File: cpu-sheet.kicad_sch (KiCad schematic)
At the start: 52 parts, among them J3 GPIO_HEADER, J4 GPIOR_HEADER, J5 USB_B_Micro, J6 PROG_CONN, U11 CH340G, U6 SRV05-4, U7 23LC1024, U8 STM32L432KC, U9 SRV05-4, Y2 32.768K, Y3 12M

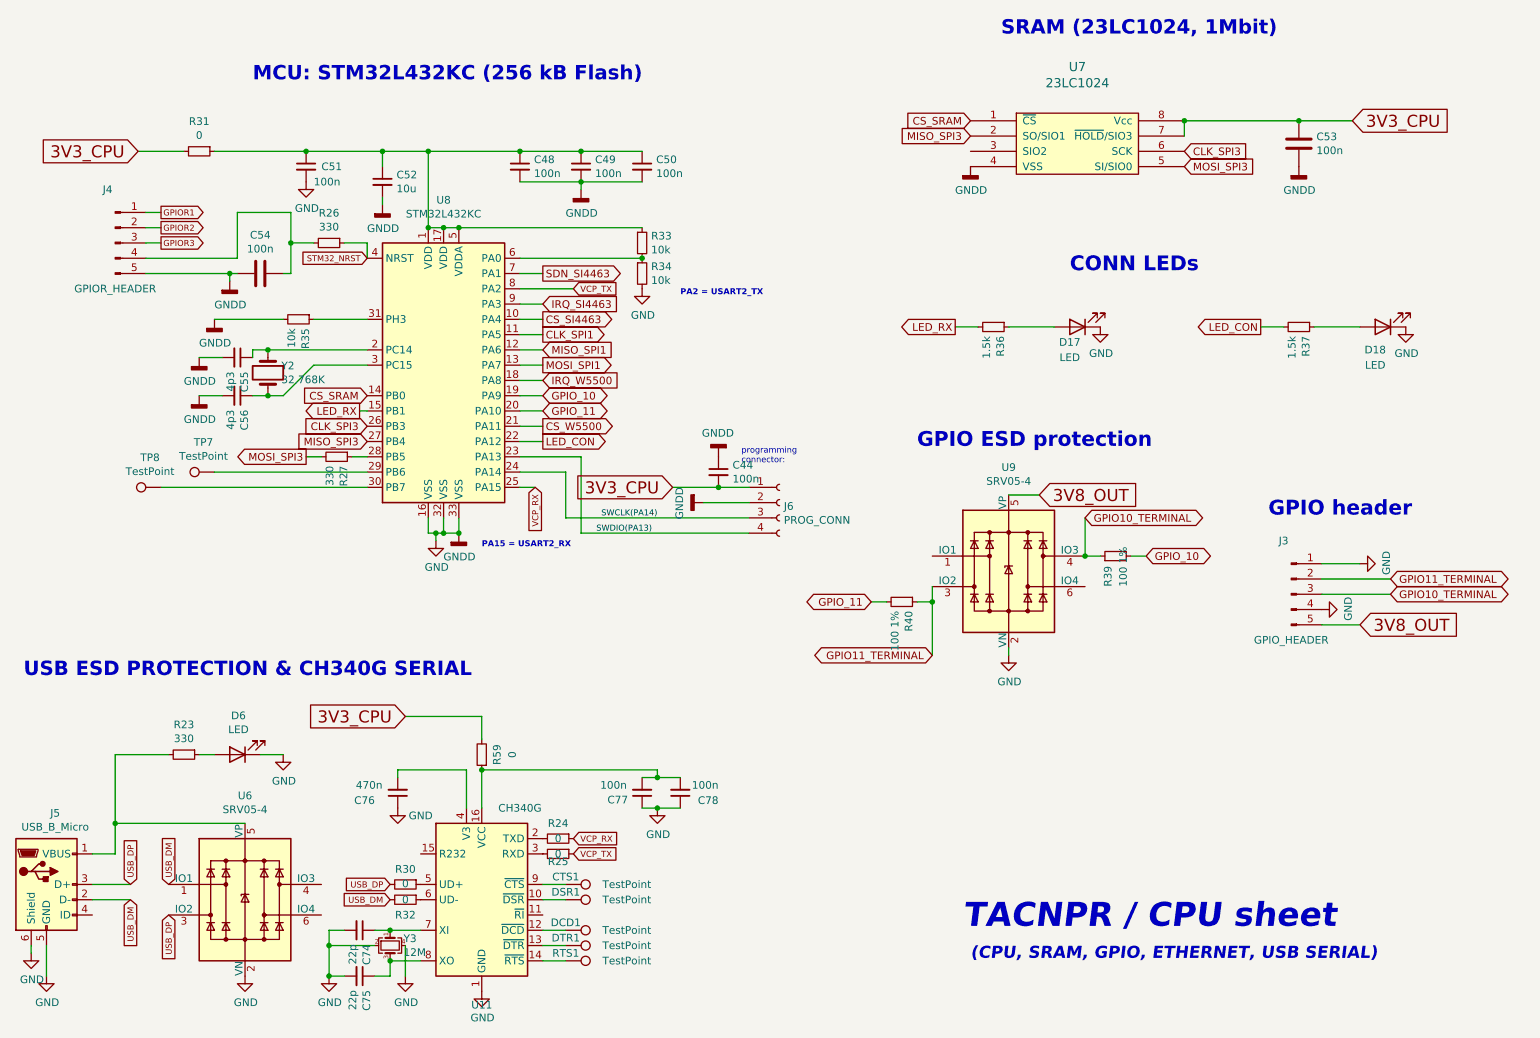
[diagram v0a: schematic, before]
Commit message: misc
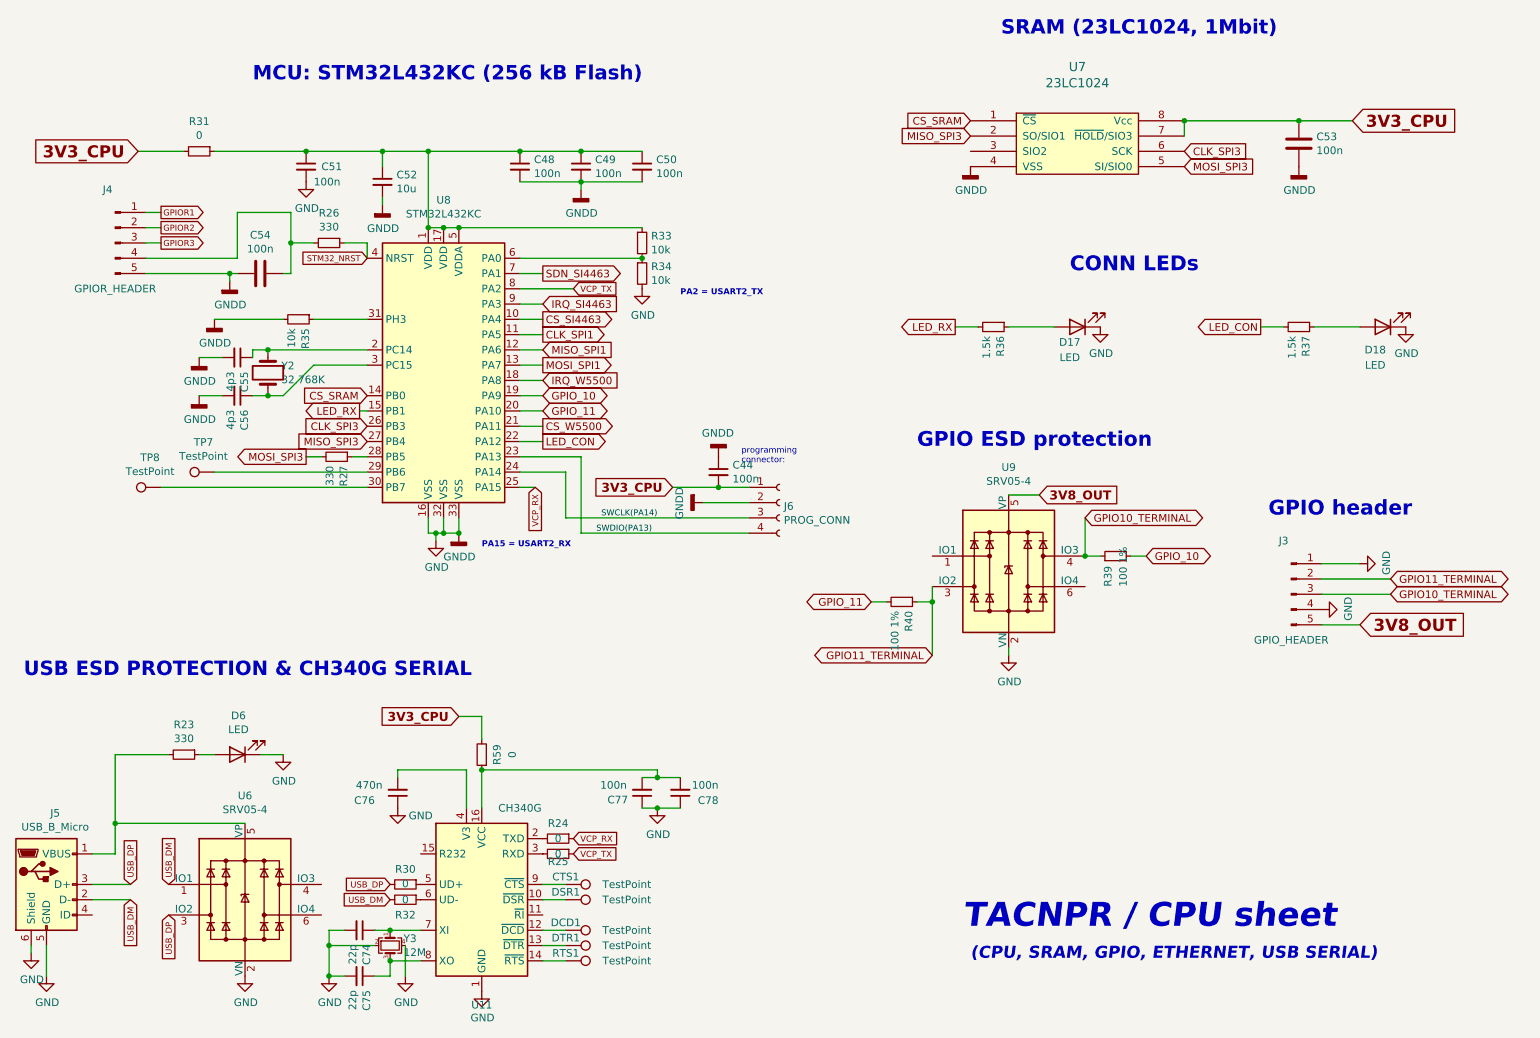
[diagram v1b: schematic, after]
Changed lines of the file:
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@@
     (stroke (width 0) (type default) (color 0 0 0 0))
   )
-  (wire (pts (xy 91.44 138.43) (xy 104.14 138.43))
+  (wire (pts (xy 100.33 138.43) (xy 104.14 138.43))
     (stroke (width 0) (type default) (color 0 0 0 0))
   )
@@
   )
   (global_label "3V3_CPU" (shape input) (at 248.92 39.37 0) (fields_autoplaced)
-    (effects (font (size 2.0066 2.0066)) (justify left))
-    (property "Intersheet References" "${INTERSHEET_REFS}" (id 0) (at 0 0 0)
-      (effects (font (size 1.27 1.27)) hide)
+    (effects (font (size 2.0066 2.0066) (thickness 0.4013) bold) (justify left))
+    (property "Intersheet References" "${INTERSHEET_REFS}" (id 0) (at 266.0792 39.1694 0)
+      (effects (font (size 2.0066 2.0066) (thickness 0.4013) bold) (justify left) hide)
     )
   )
@@
   )
   (global_label "3V8_OUT" (shape input) (at 250.19 123.19 0) (fields_autoplaced)
-    (effects (font (size 2.0066 2.0066)) (justify left))
-    (property "Intersheet References" "${INTERSHEET_REFS}" (id 0) (at 0 0 0)
-      (effects (font (size 1.27 1.27)) hide)
+    (effects (font (size 2.0066 2.0066) (thickness 0.4013) bold) (justify left))
+    (property "Intersheet References" "${INTERSHEET_REFS}" (id 0) (at 266.967 122.9894 0)
+      (effects (font (size 2.0066 2.0066) (thickness 0.4013) bold) (justify left) hide)
     )
   )
   (global_label "3V3_CPU" (shape input) (at 46.99 44.45 180) (fields_autoplaced)
-    (effects (font (size 2.0066 2.0066)) (justify right))
-    (property "Intersheet References" "${INTERSHEET_REFS}" (id 0) (at 0 0 0)
-      (effects (font (size 1.27 1.27)) hide)
+    (effects (font (size 2.0066 2.0066) (thickness 0.4013) bold) (justify right))
+    (property "Intersheet References" "${INTERSHEET_REFS}" (id 0) (at 29.8308 44.2494 0)
+      (effects (font (size 2.0066 2.0066) (thickness 0.4013) bold) (justify right) hide)
     )
   )
@@
     )
   )
-  (global_label "3V3_CPU" (shape input) (at 91.44 138.43 180) (fields_autoplaced)
-    (effects (font (size 2.0066 2.0066)) (justify right))
-    (property "Intersheet References" "${INTERSHEET_REFS}" (id 0) (at 0 0 0)
-      (effects (font (size 1.27 1.27)) hide)
+  (global_label "3V3_CPU" (shape input) (at 100.33 138.43 180) (fields_autoplaced)
+    (effects (font (size 1.5 1.5) (thickness 0.4013) bold) (justify right))
+    (property "Intersheet References" "${INTERSHEET_REFS}" (id 0) (at 87.3529 138.2425 0)
+      (effects (font (size 1.5 1.5) (thickness 0.4013) bold) (justify right) hide)
     )
   )
@@
   )
   (global_label "3V8_OUT" (shape input) (at 196.85 101.6 0) (fields_autoplaced)
-    (effects (font (size 2.0066 2.0066)) (justify left))
-    (property "Intersheet References" "${INTERSHEET_REFS}" (id 0) (at 0 0 0)
-      (effects (font (size 1.27 1.27)) hide)
+    (effects (font (size 1.5 1.5) (thickness 0.4013) bold) (justify left))
+    (property "Intersheet References" "${INTERSHEET_REFS}" (id 0) (at 209.5414 101.4125 0)
+      (effects (font (size 1.5 1.5) (thickness 0.4013) bold) (justify left) hide)
     )
   )
@@
   )
   (global_label "3V3_CPU" (shape input) (at 135.89 100.33 180) (fields_autoplaced)
-    (effects (font (size 2.0066 2.0066)) (justify right))
-    (property "Intersheet References" "${INTERSHEET_REFS}" (id 0) (at 0 0 0)
-      (effects (font (size 1.27 1.27)) hide)
-    )
-  )
+    (effects (font (size 1.5 1.5) (thickness 0.4013) bold) (justify right))
+    (property "Intersheet References" "${INTERSHEET_REFS}" (id 0) (at 122.9129 100.1425 0)
+      (effects (font (size 1.5 1.5) (thickness 0.4013) bold) (justify right) hide)
+    )
+  )
